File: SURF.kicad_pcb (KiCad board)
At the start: 2 copper layers, 33 x 30.5 mm, 33 parts, among them IC1 TPS7A0212PDBVR, IC2 TPS7A0228PDBVR, J1 Conn_01x10_Pin RIGHT, J2 Conn_01x10_Pin LEFT, J3 Conn_01x04, Q3 Q_Dual_PMOS_S1G1D2S2G2D1, U1 ESP32-S2-MINI-2

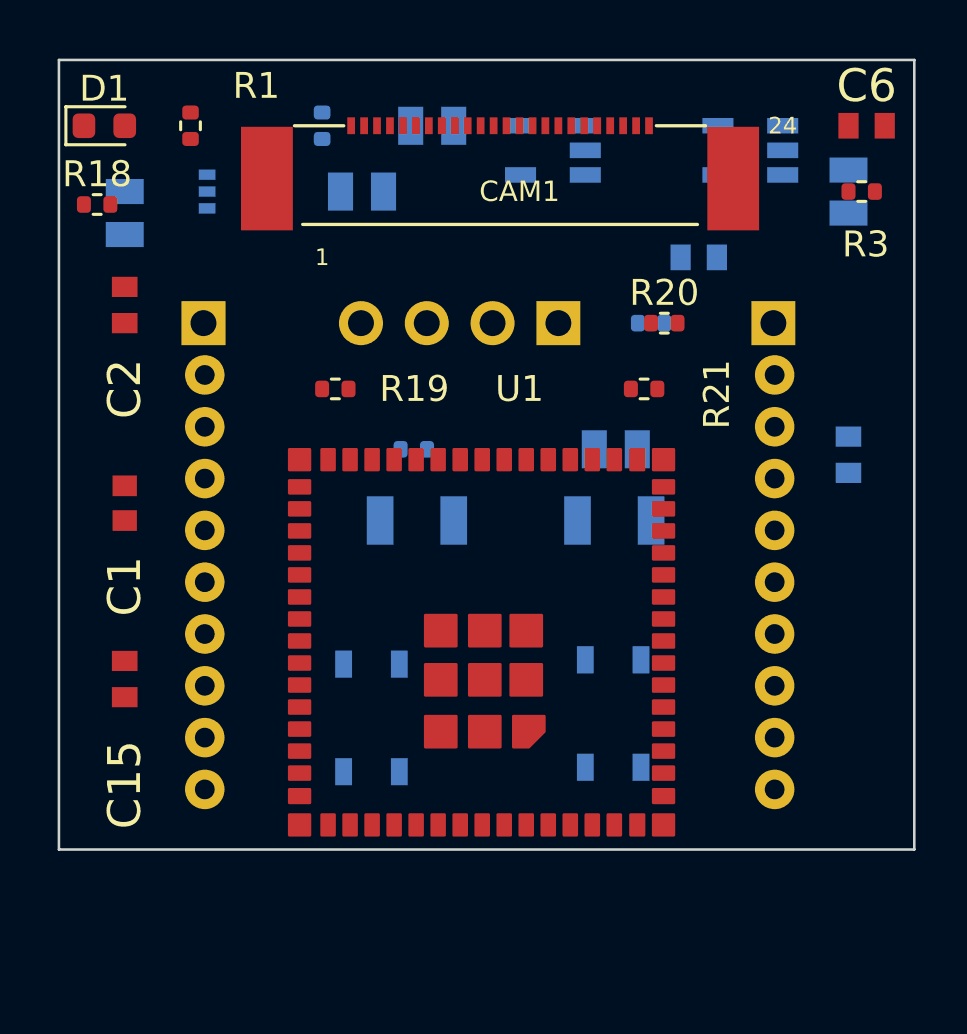
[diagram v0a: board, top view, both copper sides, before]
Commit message: new update
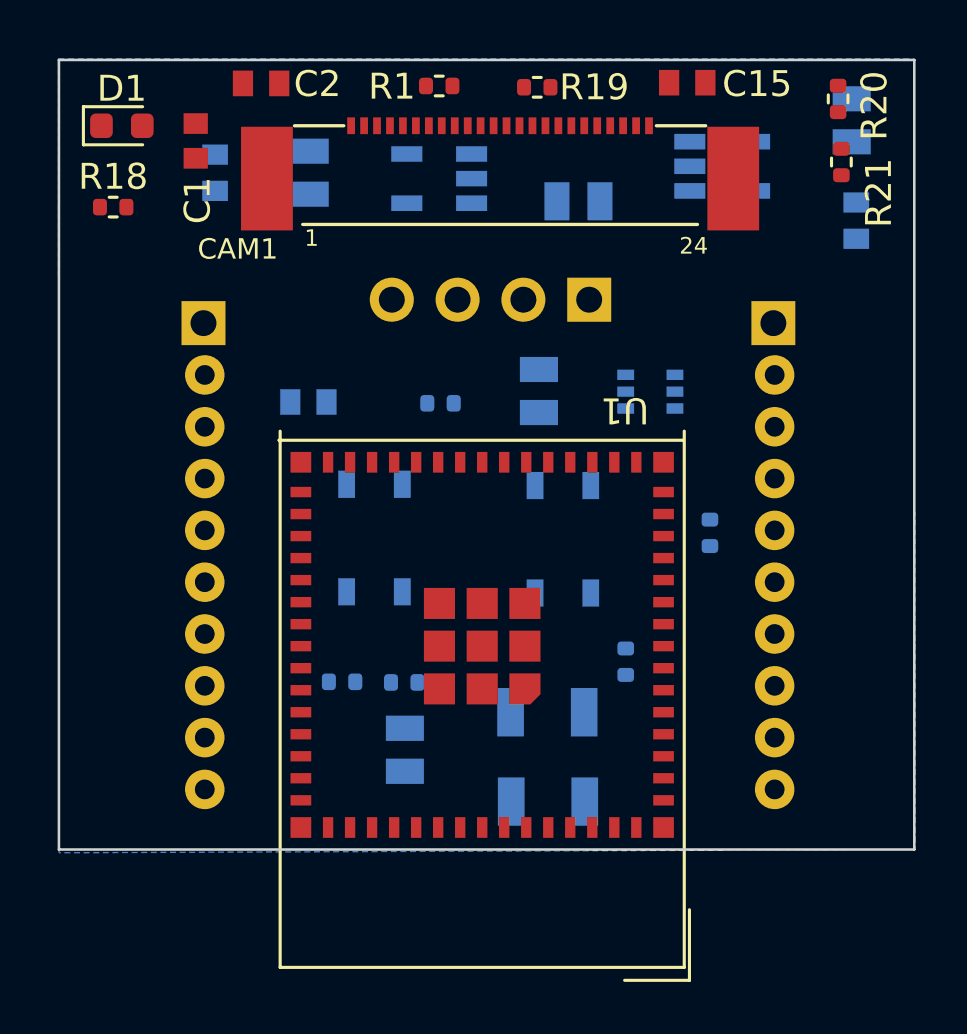
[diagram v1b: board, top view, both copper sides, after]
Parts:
- added R2: 0, Resistor_SMD:R_0402_1005Metric, B.Cu at (170.9, 95.1)
- C6, R3: moved to B.Cu
- moved C15 31.6 mm to (184.3, 72.0), turned to 180 degrees
- moved C6 24.0 mm to (169.7, 84.3), turned to 180 degrees
- moved R24 23.8 mm to (181.9, 94.3)
- moved C21 19.0 mm to (166.1, 75.5), turned to -90 degrees
- moved R3 18.2 mm to (174.8, 84.4)
- moved Q3 17.9 mm to (182.8, 83.9)
- moved C17 17.4 mm to (178.6, 83.9), turned to -90 degrees
- moved C1 14.3 mm to (165.3, 74.2), turned to -90 degrees
- moved C3 14.2 mm to (173.4, 97.8), turned to -90 degrees
- moved R19 14.0 mm to (178.5, 72.2), turned to 0 degrees
- moved IC1 12.1 mm to (174.7, 75.7)
- moved C4 12.0 mm to (178.9, 99.8)
- moved R21 11.6 mm to (190.2, 75.1), turned to 90 degrees
- moved RESET1 11.4 mm to (172.2, 89.6)
- moved R20 11.0 mm to (190.1, 72.6), turned to -90 degrees
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- renumbered S2 to BOOT1, S3 to RESET1
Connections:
- C1 pad 1: Net-(CAM1-PCLK) -> /GPIO7
- C15 pad 2: Net-(CAM1-RESET) -> /RESET
- C2 pad 1: +3V3 -> VCC
- C3 pad 1: GND -> +3V0
- C4 pad 1: +3V3 -> VCC
- C5 pad 1: +3V3 -> VCC
- CAM1 pad P$25: (no net) -> GND
- CAM1 pad P$26: (no net) -> GND
- CAM1 pad P10: (no net) -> GND
- CAM1 pad P11: (no net) -> /GPIO9
- CAM1 pad P12: (no net) -> /GPIO10
- CAM1 pad P13: (no net) -> /GPIO11
- CAM1 pad P14: (no net) -> DOVDD
- CAM1 pad P15: (no net) -> DVDD
- CAM1 pad P16: (no net) -> /GPIO12
- CAM1 pad P17: (no net) -> /PWDN
- CAM1 pad P18: (no net) -> /GPIO13
- CAM1 pad P19: (no net) -> /RESET
- CAM1 pad P20: (no net) -> /TWI_SCK
- CAM1 pad P21: (no net) -> AVDD
- CAM1 pad P22: (no net) -> /TWI_SDA
- CAM1 pad P23: (no net) -> GND
- CAM1 pad P3: (no net) -> /GPIO2
- CAM1 pad P4: (no net) -> /GPIO3
- CAM1 pad P5: (no net) -> /GPIO4
- CAM1 pad P6: (no net) -> /GPIO5
- CAM1 pad P7: (no net) -> /GPIO6
- CAM1 pad P8: (no net) -> /GPIO7
- CAM1 pad P9: (no net) -> /GPIO8
- J3 pad 3: Net-(J3-Pin_3) -> /TXD0
- Q3 pad 2: Net-(Q3A-G) -> unconnected-(Q3A-G-Pad2)
- R1 pad 1: Net-(CAM1-PWDN) -> /PWDN
- R19 pad 1: Net-(CAM1-RESET) -> /RESET
- R20 pad 1: Net-(CAM1-SIO_C) -> /TWI_SCK
- R21 pad 1: Net-(CAM1-SIO_D) -> /TWI_SDA
- R23 pad 1: VCC -> Net-(IC1-IN)
- R23 pad 2: Net-(Q3A-G) -> Net-(R23-Pad2)
- R24 pad 1: Net-(Q3A-G) -> Net-(R23-Pad2)
- RESET1 pad 3: GND -> Net-(RESET1-COM_1)
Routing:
- added copper zone on B.Cu, net GND
